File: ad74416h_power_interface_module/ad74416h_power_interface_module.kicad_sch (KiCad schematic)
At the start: 18 parts, among them J1 CLP-133-02-G-D-BE, J2 TBP02R1-381-02BE, J3 FW-04-05-G-D-470-160, J4 CLP-117-02-G-D-BE, J5 FW-04-05-F-D-248-160, J6 TBP02R1-381-02BE

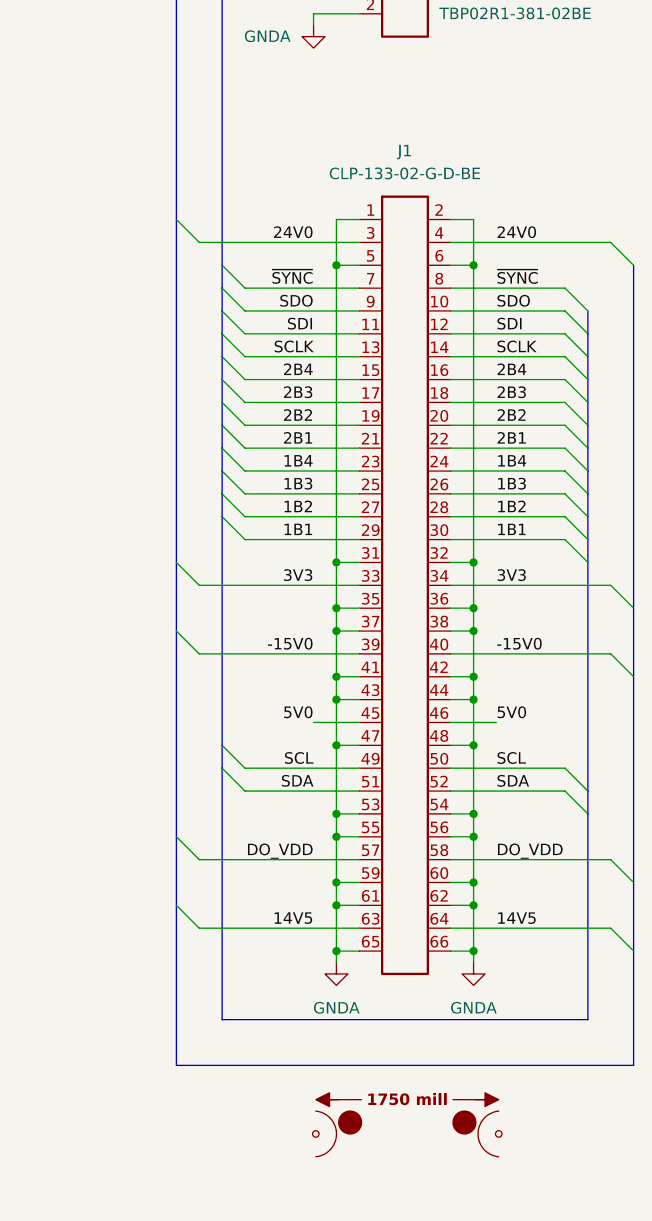
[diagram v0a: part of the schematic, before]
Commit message: backup
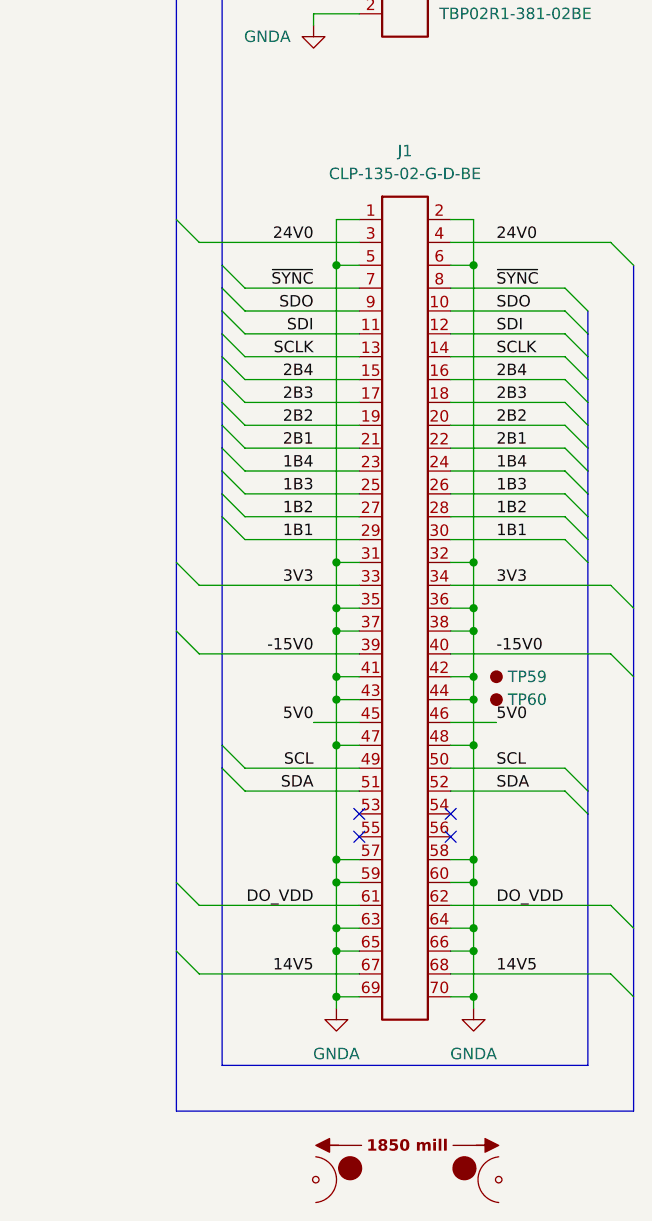
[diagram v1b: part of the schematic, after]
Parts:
- added TP59, TP60: TestPoint, test_point_footprints:TestPoint_THTPad_Castelated, symbol UNITED_TEST_POINTS:TestPoint_Castelated_v2
- J1: value CLP-133-02-G-D-BE -> CLP-135-02-G-D-BE; footprint connector_footprints:CLP-133-02-G-D-BE -> connector_footprints:CLP-135-02-G-D-BE; symbol CONNECTORS_CLP-1xx-02-G-D-BE_DATA_BASE:J_CLP-133-02-G-D-BE -> CONNECTORS_CLP-1xx-02-G-D-BE_DATA_BASE:J_CLP-135-02-G-D-BE; MPN CLP-133-02-G-D-BE -> CLP-135-02-G-D-BE; Pin Count 33 -> 35; Symbol Name J_CLP-133-02-G-D-BE -> J_CLP-135-02-G-D-BE; Trustedparts Search https://www.trustedparts.com/en/search/CLP-133-02-G-D-BE -> https://www.trustedparts.com/en/search/CLP-135-02-G-D-BE
- MB1: value mouse-bite-50mil-1750mil -> mouse-bite-50mil-1850mil; footprint mouse_bite_footprints:mouse-bite-50mil-1750mil -> mouse_bite_footprints:mouse-bite-50mil-1850mil; symbol UNITED_MOUSE_BITES_DATA_BASE:mouse-bite-50mil-1750mil -> UNITED_MOUSE_BITES_DATA_BASE:mouse-bite-50mil-1850mil
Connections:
- net 14V5: now also J1.67, J1.68; no longer J1.63, J1.64
- net DO_VDD: now also J1.61, J1.62; no longer J1.57, J1.58
- net GNDA: now also J1.57, J1.58, J1.63, J1.64, J1.69, J1.70; no longer J1.53, J1.54, J1.55, J1.56, J1.61, J1.62
- no-connect marks 0 -> 4
